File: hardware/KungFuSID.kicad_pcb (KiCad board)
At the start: 4 copper layers, 21 x 39 mm, 33 parts, among them J1 SWD, U1 AMS1117-3.3, U2 C64-SID-Socket-hackup, U3 GD32F405RGT6, U4 LM321, Y1 8MHz

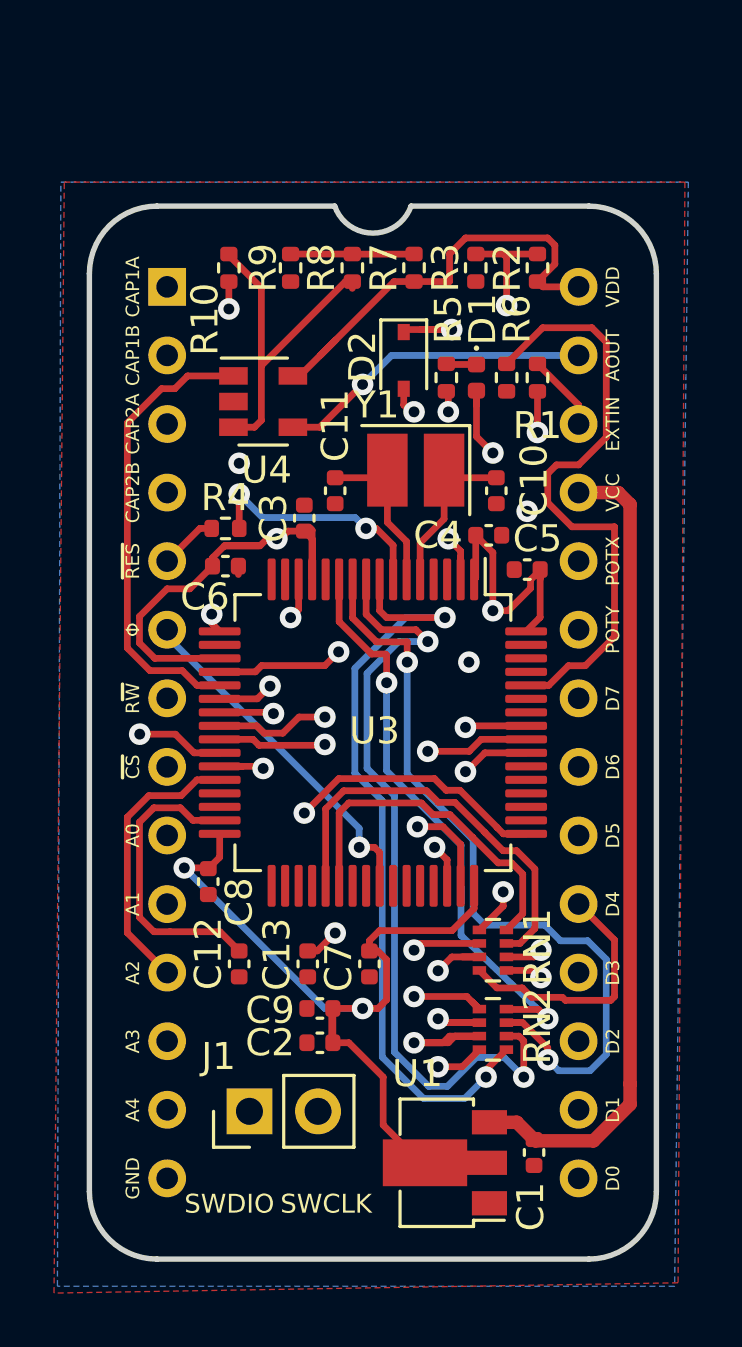
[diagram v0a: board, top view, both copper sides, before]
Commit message: Attempts to make Potxy(please still use release version) Update of hardware files
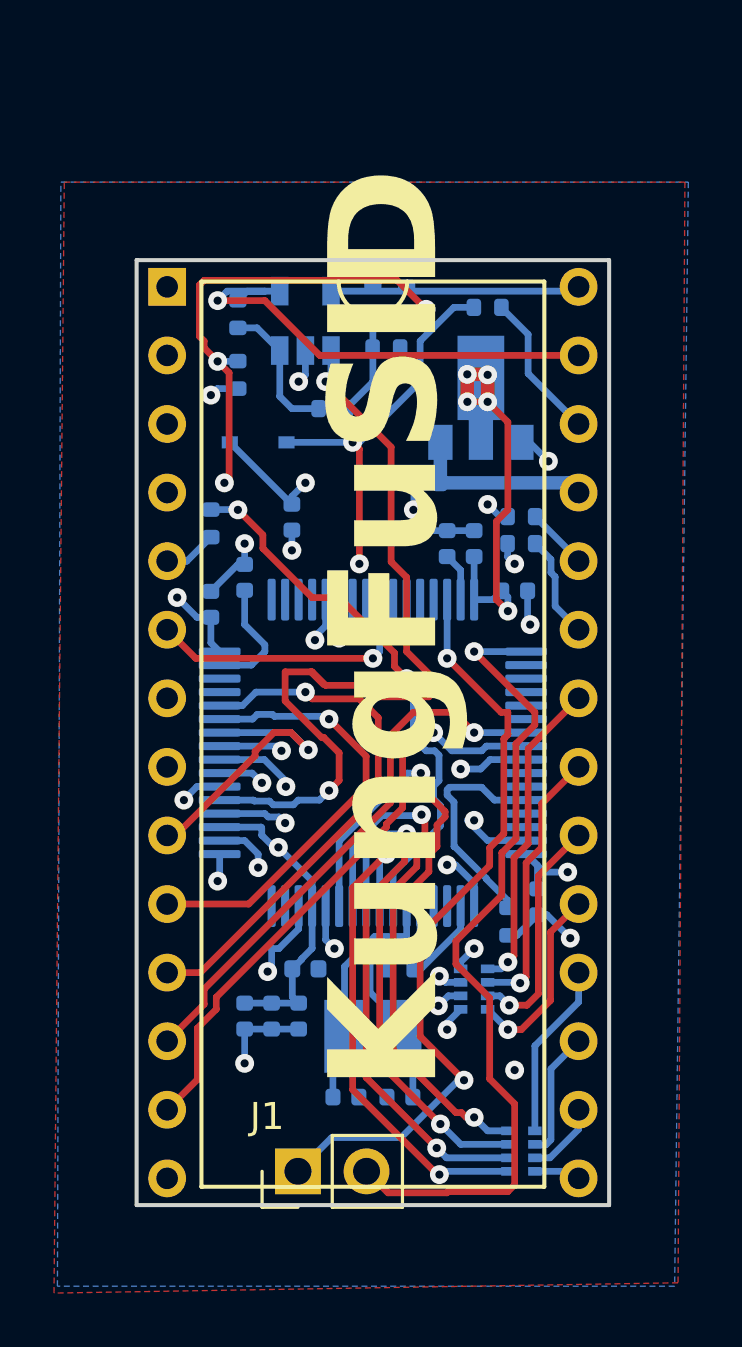
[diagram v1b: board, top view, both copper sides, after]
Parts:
- added R11: 470, Resistor_SMD:R_0402_1005Metric, B.Cu at (80.5, 91.5)
- added R12: 470, Resistor_SMD:R_0402_1005Metric, B.Cu at (80.5, 92.5)
- C1, C10, C11, C12, C13, C2, C3, C4, C5, C6, C7, C8, C9, D1, D2, R1, R2, R3, R4, R5, R6, R7, R8, RN1, RN2, U1, U3, U4, Y1: moved to B.Cu
- R10: value 2k -> 0; moved to B.Cu
- R9: value 470 -> 33; moved to B.Cu
- moved U1 28.4 mm to (79.0, 87.1), turned to 90 degrees
- moved C1 25.1 mm to (77.0, 90.2), turned to 180 degrees
- moved D1 22.8 mm to (72.5, 108.2), turned to 180 degrees
- moved C10 22.7 mm to (76.0, 113.0), turned to 0 degrees
- moved C11 22.5 mm to (74.0, 113.0), turned to 0 degrees
- moved R5 22.0 mm to (76.0, 108.2), turned to 180 degrees
- moved Y1 21.0 mm to (75.0, 110.8)
- moved R6 20.2 mm to (80.0, 106.5)
- moved C13 16.4 mm to (77.8, 92.5), turned to 90 degrees
- moved C12 14.3 mm to (70.2, 93.8), turned to -90 degrees
- moved C8 12.2 mm to (81.1, 105.8)
- moved C5 11.8 mm to (69.0, 94.8), turned to 90 degrees
- moved C6 10.8 mm to (80.2, 94.2)
- moved R3 9.66 mm to (70.0, 86.2)
- moved C4 7.32 mm to (72.0, 91.5), turned to -90 degrees
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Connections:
- U2 pad 1: Net-(U2-Pad1) -> unconnected-(U2-CAP1A-Pad1)
- U2 pad 2: Net-(U2-Pad2) -> unconnected-(U2-CAP1B-Pad2)
- U2 pad 23: /POT_Y -> /I_P_Y
- U2 pad 24: /POT_X -> /I_P_X
- U2 pad 3: Net-(U2-Pad3) -> unconnected-(U2-CAP2A-Pad3)
- U2 pad 4: Net-(U2-Pad4) -> unconnected-(U2-CAP2B-Pad4)
- U3 pad 15: Net-(U3-Pad15) -> unconnected-(U3-PA1-Pad15)
- U3 pad 16: Net-(U3-Pad16) -> unconnected-(U3-PA2-Pad16)
- U3 pad 29: Net-(U3-Pad29) -> unconnected-(U3-PB10-Pad29)
- U3 pad 3: Net-(U3-Pad3) -> unconnected-(U3-PC14-Pad3)
- U3 pad 30: Net-(U3-Pad30) -> unconnected-(U3-PB11-Pad30)
- U3 pad 33: Net-(U3-Pad33) -> unconnected-(U3-PB12-Pad33)
- U3 pad 34: Net-(U3-Pad34) -> unconnected-(U3-PB13-Pad34)
- U3 pad 35: Net-(U3-Pad35) -> unconnected-(U3-PB14-Pad35)
- U3 pad 36: Net-(U3-Pad36) -> unconnected-(U3-PB15-Pad36)
- U3 pad 39: Net-(U3-Pad39) -> unconnected-(U3-PC8-Pad39)
- U3 pad 4: Net-(U3-Pad4) -> unconnected-(U3-PC15-Pad4)
- U3 pad 40: Net-(U3-Pad40) -> unconnected-(U3-PC9-Pad40)
- U3 pad 42: Net-(U3-Pad42) -> unconnected-(U3-PA9-Pad42)
- U3 pad 43: Net-(U3-Pad43) -> unconnected-(U3-PA10-Pad43)
- U3 pad 44: Net-(U3-Pad44) -> unconnected-(U3-PA11-Pad44)
- U3 pad 45: Net-(U3-Pad45) -> unconnected-(U3-PA12-Pad45)
- U3 pad 50: Net-(U3-Pad50) -> unconnected-(U3-PA15-Pad50)
- U3 pad 51: Net-(U3-Pad51) -> unconnected-(U3-PC10-Pad51)
- U3 pad 52: Net-(U3-Pad52) -> unconnected-(U3-PC11-Pad52)
- U3 pad 53: Net-(U3-Pad53) -> unconnected-(U3-PC12-Pad53)
- U3 pad 54: Net-(U3-Pad54) -> unconnected-(U3-PD2-Pad54)
- U3 pad 58: Net-(U3-Pad58) -> unconnected-(U3-PB6-Pad58)
- U3 pad 59: Net-(U3-Pad59) -> unconnected-(U3-PB7-Pad59)
- U3 pad 61: Net-(U3-Pad61) -> unconnected-(U3-PB8-Pad61)
- U3 pad 62: Net-(U3-Pad62) -> unconnected-(U3-PB9-Pad62)
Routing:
- net GND: track 0.31 -> 25.4 mm, vias 3 -> 14
- net +5V: track 30.4 -> 6.80 mm
- net +3V3: track 102.0 -> 81.4 mm, vias 6 -> 10
- net /~{CS}: track 15.4 -> 34.2 mm
- net /BOOT0: track 22.7 -> 8.48 mm
- net /SPECIAL: track 17.2 -> 30.8 mm, vias 0 -> 2
- net /~{RST}: track 9.02 -> 20.4 mm
- net /SWDIO: track 17.8 -> 28.4 mm, vias 1 -> 2
- net /EXT_IN: track 19.7 -> 30.3 mm
- net /D0: track 28.8 -> 18.4 mm
- net /CD1: track 12.9 -> 2.78 mm, vias 1 -> 0
- net /SWCLK: track 21.0 -> 30.7 mm
- net /A2: track 10.4 -> 19.9 mm, vias 0 -> 1
- net /D1: track 29.3 -> 20.0 mm
- net /VDD_ADC: track 26.6 -> 35.2 mm, vias 2 -> 4
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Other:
- board size 21 x 39 mm -> 17.5 x 35 mm
- board text added: "KungFuSID"
- board text removed: "SWCLK"
- board text removed: "SWDIO"
